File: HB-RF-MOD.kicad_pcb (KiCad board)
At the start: 2 copper layers, 36.2 x 65 mm, 25 parts, among them J1 RPi Header, J2 RGB, Q1 BC847, SW1 Button, U1 TRX2-TIF, U2 RX8130-CE, U3 3V3LDO

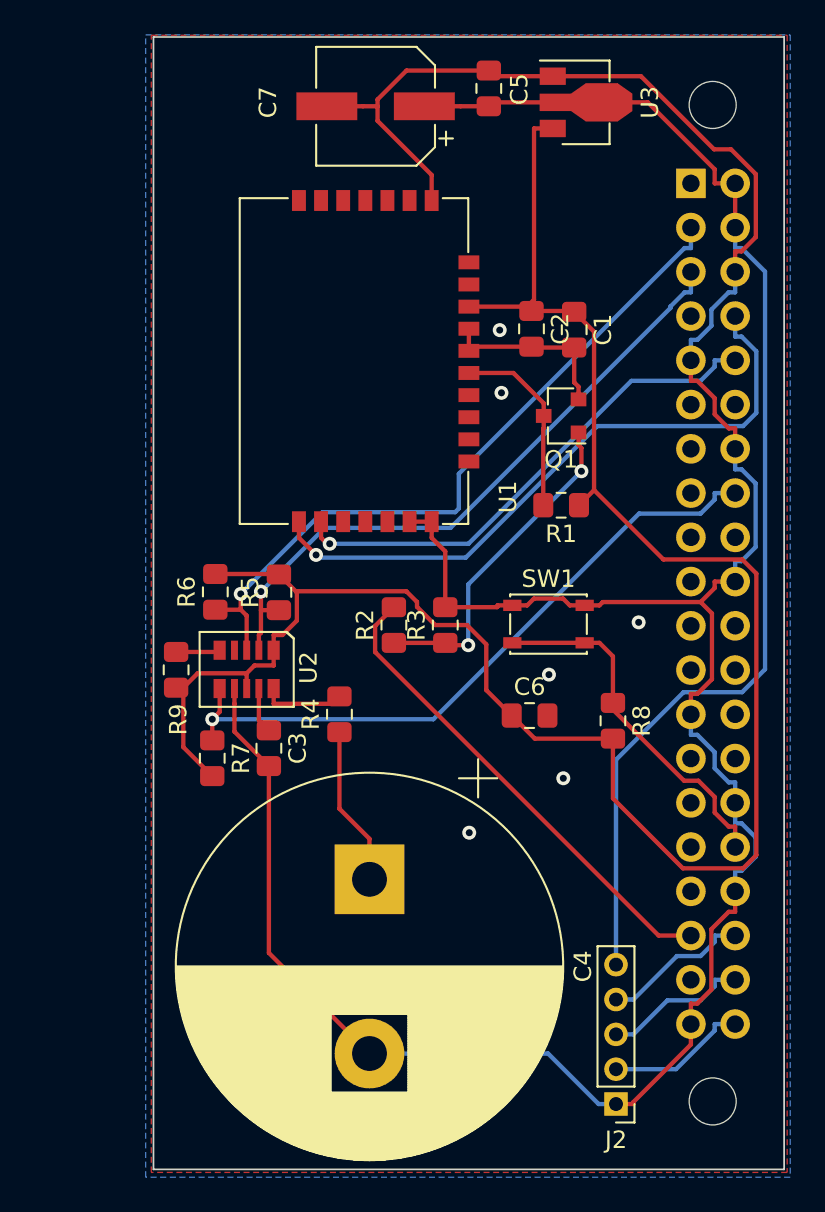
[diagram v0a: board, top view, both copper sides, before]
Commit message: update
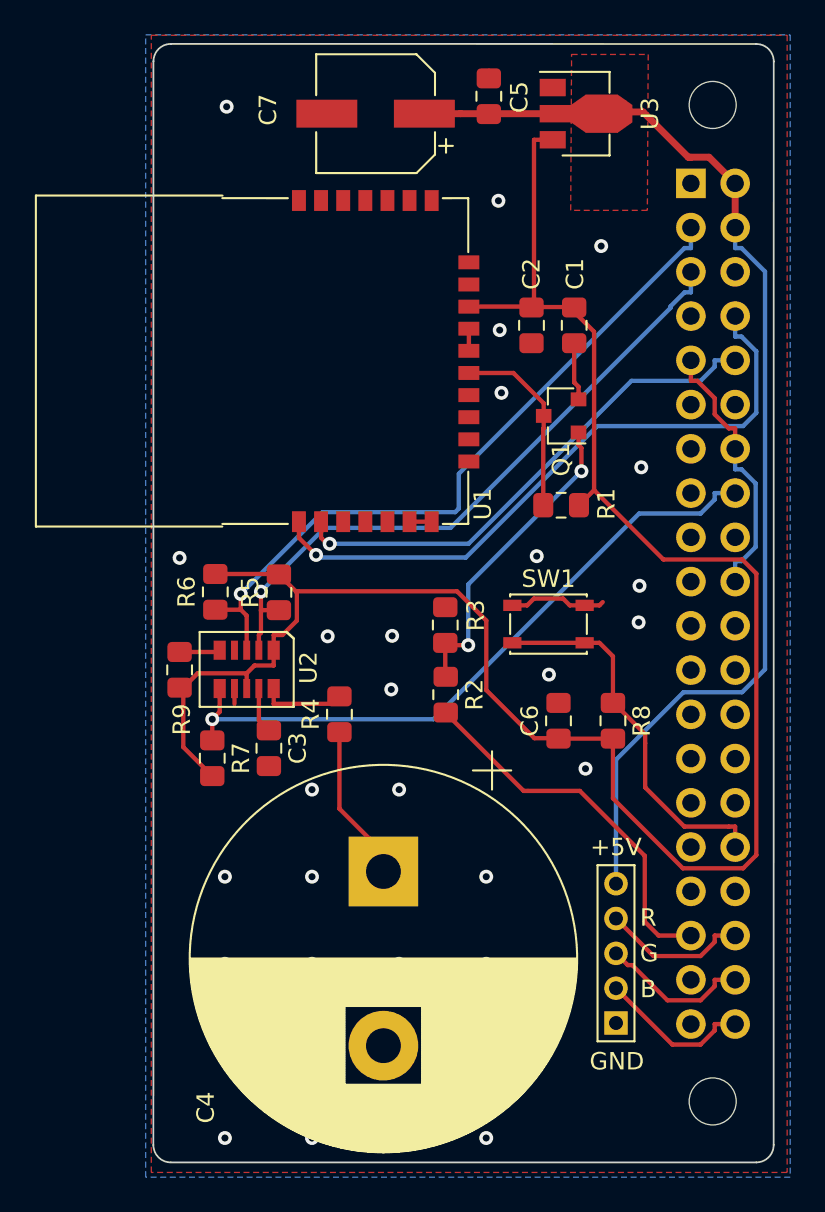
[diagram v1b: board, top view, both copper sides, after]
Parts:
- moved R2 4.98 mm to (177.7, 94.5), turned to 270 degrees
- moved J2 4.65 mm to (187.4, 113.4)
- moved C6 1.69 mm to (184.2, 96.0), turned to 90 degrees
- moved C4 0.92 mm to (174.1, 104.7)
- moved U3 0.65 mm to (185.3, 61.2)
- moved C5 0.45 mm to (180.2, 60.2)
- moved C7 0.43 mm to (173.7, 61.2)
- moved C1 0.25 mm to (185.1, 73.3)
- moved R9 0.20 mm to (162.4, 93.1)
- moved C2 0.20 mm to (182.6, 73.3)
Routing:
- net GND: track 174.1 -> 28.2 mm, vias 6 -> 30
- net RESET: track 27.9 -> 21.5 mm
- net +5V: track 71.6 -> 65.9 mm
- net BUTTON: track 20.7 -> 22.0 mm
- net Net-(Q1-Pad1): track 19.3 -> 18.2 mm
- net Net-(J1-Pad40): track 8.13 -> 8.88 mm
- added copper zone on F.Cu, net +5V
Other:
- board size 36.2 x 65 mm -> 35.6 x 64.2 mm
- board text added: "+5V"
- board text added: "B"
- board text added: "G"
- board text added: "GND"
- board text added: "R"
